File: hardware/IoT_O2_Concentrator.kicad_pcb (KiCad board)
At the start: 2 copper layers, 92.8 x 88.4 mm, 17 parts, among them J1 5V_SUPPLY_BUCK_OUT, J10 12V_SUPPLY_BUCK_IN, J11 O2_VCC_SELECTOR, J12 BOX_SWITCH, J13 AC-DC_MODULE, J2 BUZZER, J3 O2_SENSOR, J4 GPIOs, J5 RELAY, J6 LCD_20x04, J7 SIM_GSM_EVB, J8 POTENTIOMETER, J9 SUPPLY

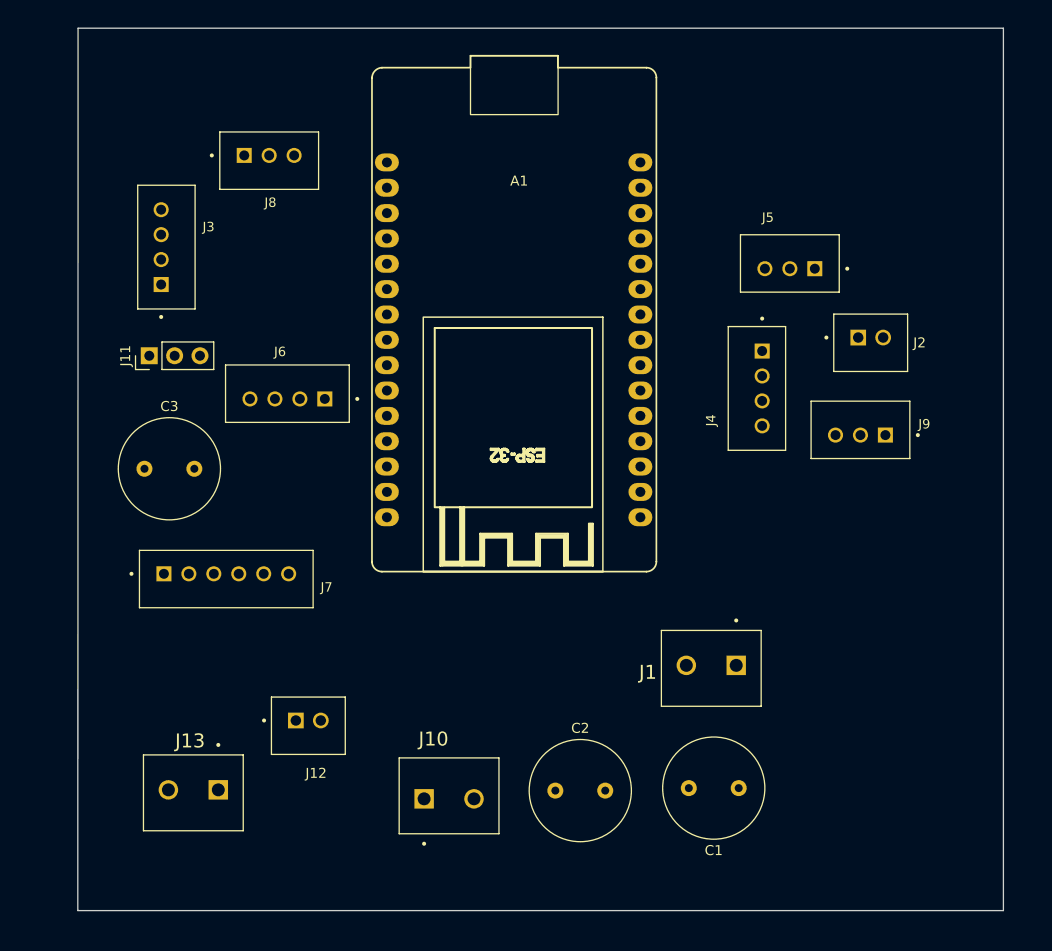
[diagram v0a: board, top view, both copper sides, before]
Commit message: Finishing the routing
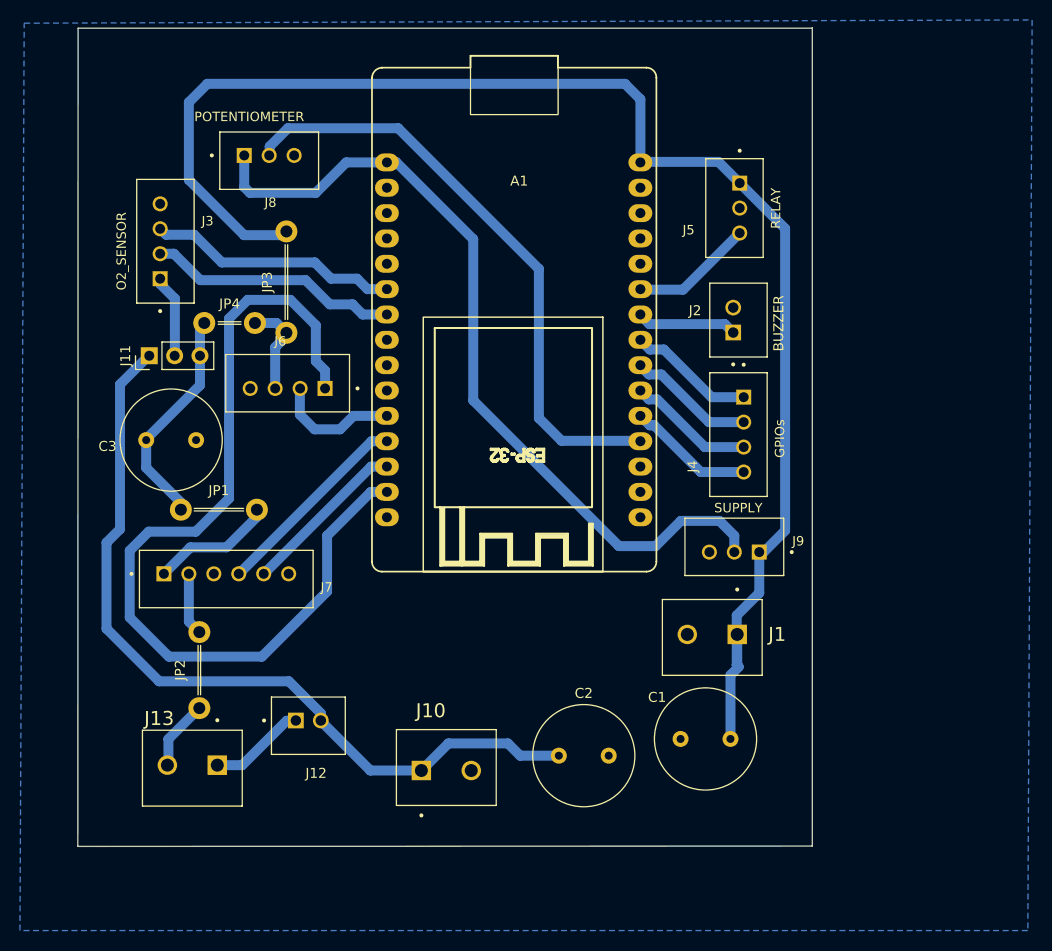
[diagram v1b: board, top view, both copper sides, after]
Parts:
- added JP1: 5V_JUMPER, PCM_Jumper_AKL:Jumper_P7.62mm_D1.2mm, F.Cu at (122.7, 88.2)
- added JP2: GND_JUMPER, PCM_Jumper_AKL:Jumper_P7.62mm_D1.2mm, F.Cu at (124.5, 108.1)
- added JP3: 5V_JUMPER, PCM_Jumper_AKL:Jumper_P10.16mm_D1.2mm, F.Cu at (133.3, 70.5)
- added JP4: 5V_JUMPER, PCM_Jumper_AKL:Jumper_P5.08mm_D1.2mm, F.Cu at (125.0, 69.5)
- moved J9 17.2 mm to (178.2, 92.0)
- moved J2 13.4 mm to (178.6, 69.2), turned to -90 degrees
- moved J5 7.85 mm to (178.2, 58.0), turned to 90 degrees
- moved C1 4.99 mm to (177.8, 111.2)
- moved J4 4.98 mm to (178.6, 80.7)
- moved C2 3.52 mm to (160.6, 112.9)
- moved J1 3.10 mm to (178.4, 100.8)
- moved C3 2.88 mm to (119.2, 81.3)
- moved J10 2.85 mm to (146.8, 114.4)
- moved J13 2.48 mm to (126.3, 113.8)
- moved J6 1.05 mm to (133.4, 75.6)
- moved J3 0.60 mm to (121.2, 61.4)
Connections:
- J4 pad 2: /GPIO32 -> /GPIO33
- J4 pad 3: /GPIO33 -> /GPIO32
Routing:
- net /5V_VCC: track 0.00 -> 191.7 mm
- net /SCL_22: track 0.00 -> 91.6 mm
- net /12V_VCC: track 0.00 -> 82.4 mm
- net /3V3_VCC: track 0.00 -> 82.3 mm
- net /POT_34: track 0.00 -> 60.6 mm
- net /O2_RXD: track 0.00 -> 25.2 mm
- net /O2_TXD: track 0.00 -> 25.2 mm
- net /SIM_TXD: track 0.00 -> 20.4 mm
- net /SIM_RXD: track 0.00 -> 16.8 mm
- net GND: track 0.00 -> 13.3 mm
- net /GPIO25: track 0.00 -> 12.8 mm
- net /GPIO32: track 0.00 -> 12.8 mm
- net /GPIO33: track 0.00 -> 12.8 mm
- net /GPIO35: track 0.00 -> 12.7 mm
- net /SDA_21: track 0.00 -> 12.5 mm
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- added copper zone on B.Cu, net GND
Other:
- board size 92.8 x 88.4 mm -> 73.6 x 82 mm
